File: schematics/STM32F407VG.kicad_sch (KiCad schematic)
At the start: 35 parts, among them Q1 MMBT3904, Q2 MMBT3904, SW1 SW_DPST_x2, U5 STM32F407VGTx, X1 8MHz

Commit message: Было еще что-то 1206
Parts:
- R14, R15, R17, R18, R19, R20, R21, R22, R23: footprint Resistor_SMD:R_1206_3216Metric_Pad1.30x1.75mm_HandSolder -> Resistor_SMD:R_0805_2012Metric
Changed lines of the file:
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@@
 			)
 		)
-		(property "Footprint" "Resistor_SMD:R_1206_3216Metric_Pad1.30x1.75mm_HandSolder"
+		(property "Footprint" "Resistor_SMD:R_0805_2012Metric"
 			(at 143.51 101.092 90)
 			(effects
@@
 			)
 		)
-		(property "Footprint" "Resistor_SMD:R_1206_3216Metric_Pad1.30x1.75mm_HandSolder"
+		(property "Footprint" "Resistor_SMD:R_0805_2012Metric"
 			(at 143.51 111.252 90)
 			(effects
@@
 			)
 		)
-		(property "Footprint" "Resistor_SMD:R_1206_3216Metric_Pad1.30x1.75mm_HandSolder"
+		(property "Footprint" "Resistor_SMD:R_0805_2012Metric"
 			(at 143.51 103.632 90)
 			(effects
@@
 			)
 		)
-		(property "Footprint" "Resistor_SMD:R_1206_3216Metric_Pad1.30x1.75mm_HandSolder"
+		(property "Footprint" "Resistor_SMD:R_0805_2012Metric"
 			(at 143.51 106.172 90)
 			(effects
@@
 			)
 		)
-		(property "Footprint" "Resistor_SMD:R_1206_3216Metric_Pad1.30x1.75mm_HandSolder"
+		(property "Footprint" "Resistor_SMD:R_0805_2012Metric"
 			(at 55.88 111.252 90)
 			(effects
@@
 			)
 		)
-		(property "Footprint" "Resistor_SMD:R_1206_3216Metric_Pad1.30x1.75mm_HandSolder"
+		(property "Footprint" "Resistor_SMD:R_0805_2012Metric"
 			(at 143.51 55.372 90)
 			(effects
@@
 			)
 		)
-		(property "Footprint" "Resistor_SMD:R_1206_3216Metric_Pad1.30x1.75mm_HandSolder"
+		(property "Footprint" "Resistor_SMD:R_0805_2012Metric"
 			(at 55.88 108.712 90)
 			(effects
@@
 			)
 		)
-		(property "Footprint" "Resistor_SMD:R_1206_3216Metric_Pad1.30x1.75mm_HandSolder"
+		(property "Footprint" "Resistor_SMD:R_0805_2012Metric"
 			(at 143.51 108.712 90)
 			(effects
@@
 			)
 		)
-		(property "Footprint" "Resistor_SMD:R_1206_3216Metric_Pad1.30x1.75mm_HandSolder"
+		(property "Footprint" "Resistor_SMD:R_0805_2012Metric"
 			(at 143.51 52.832 90)
 			(effects

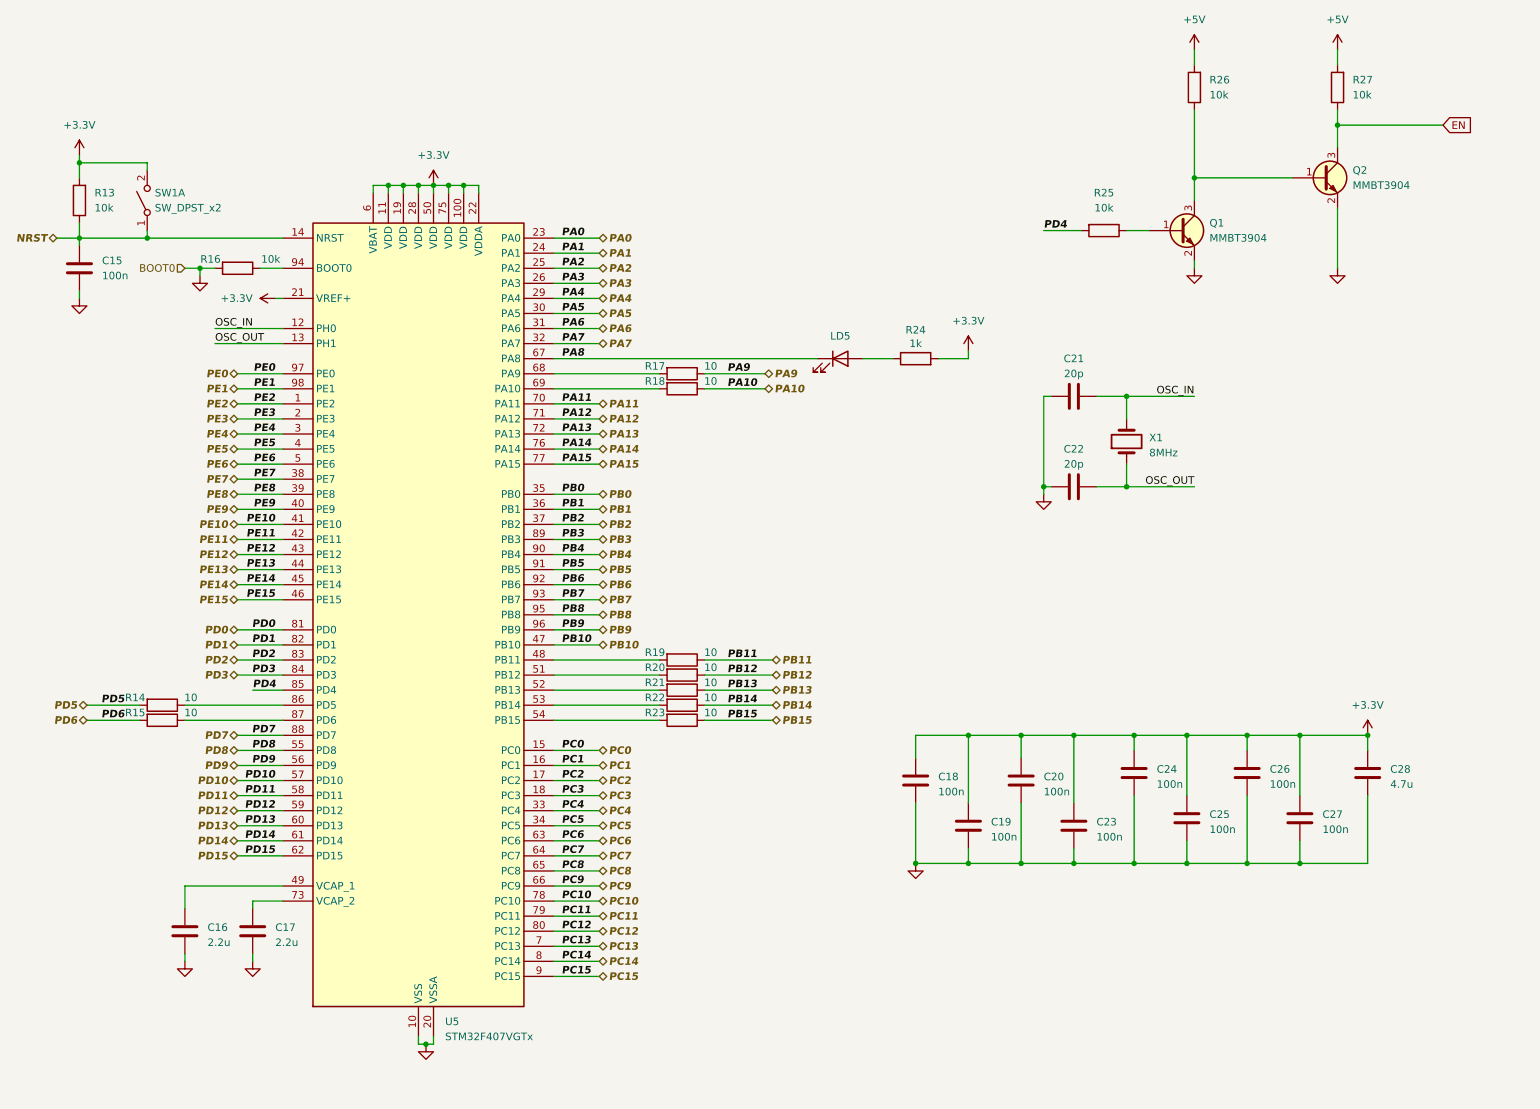
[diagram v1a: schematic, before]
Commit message: Правки схем, возможно что-то было не корректно выбрано
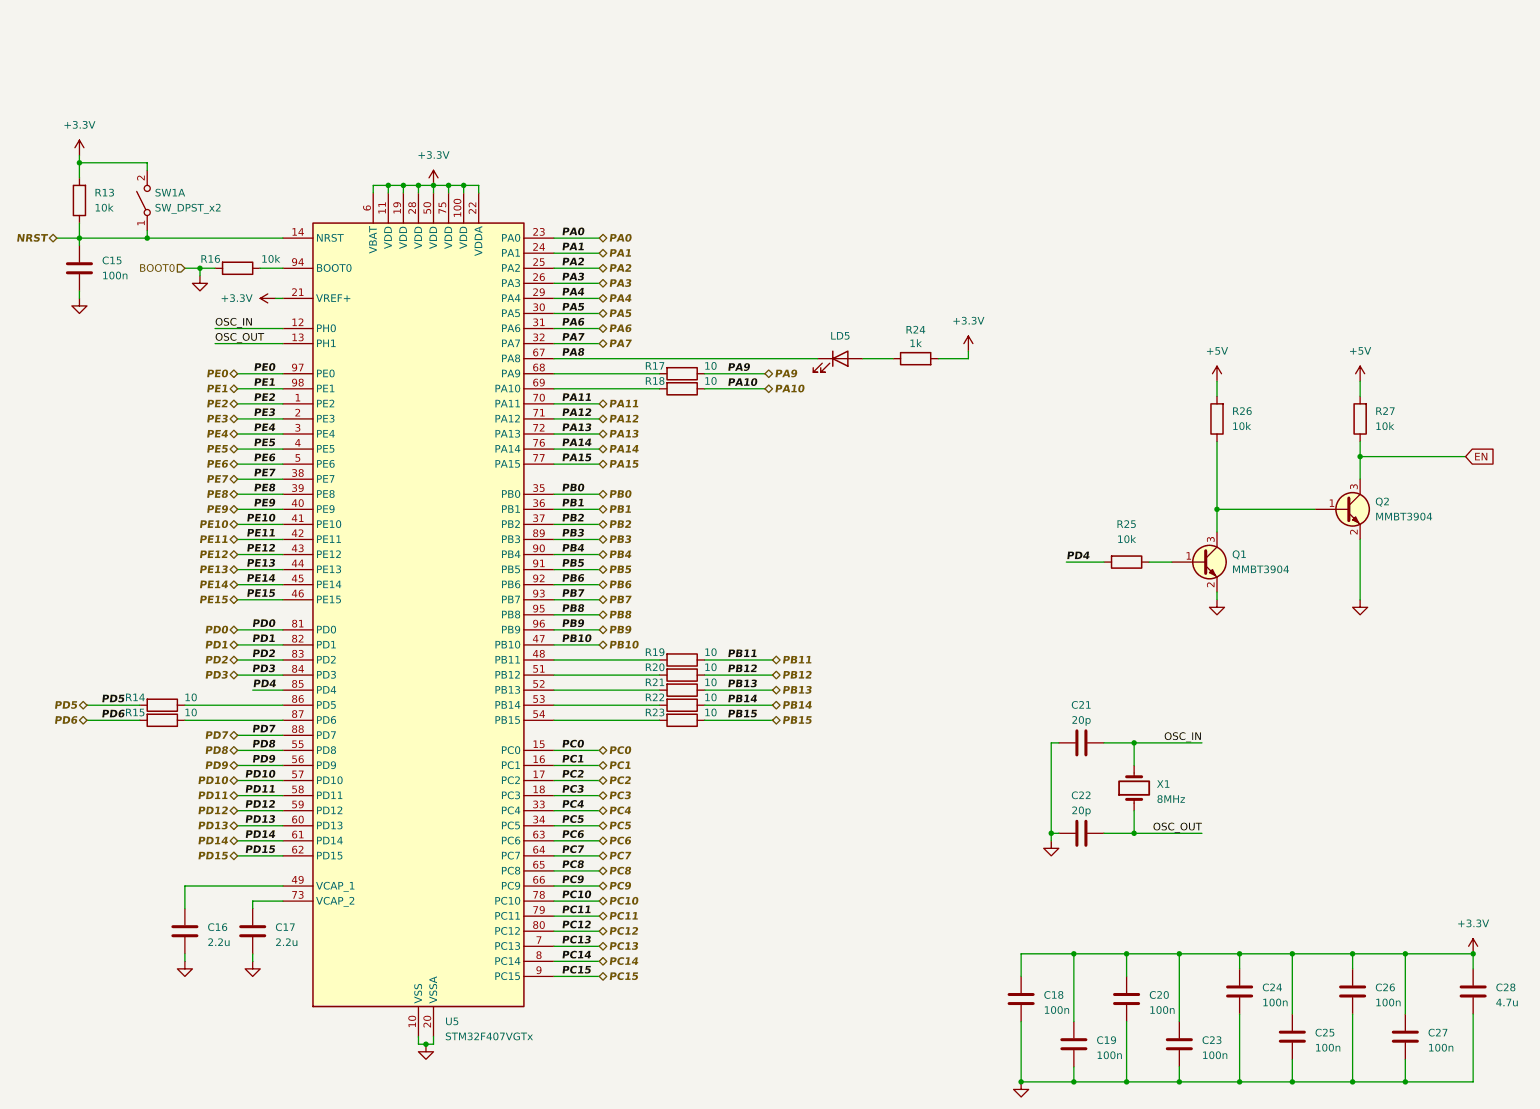
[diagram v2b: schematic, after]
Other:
- moved on the sheet: C18, C19, C20, C21, C22, C23, C24, C25, C26, C27, C28, Q1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
